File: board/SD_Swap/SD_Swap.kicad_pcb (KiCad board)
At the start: 4 copper layers, 32 x 27 mm, 44 parts, among them J1 USB_C, Q1 Q_Dual_PNP_PNP_E1B1C2E2B2C1, U1 74LVC2G14, U2 RTS5306E, U3 PCB_SD, U4 93AAxxAT, U5 TS3A27518ERTW, U6 SD_SOCKET, U7 AZ1117-3.3, Y1 12MHz

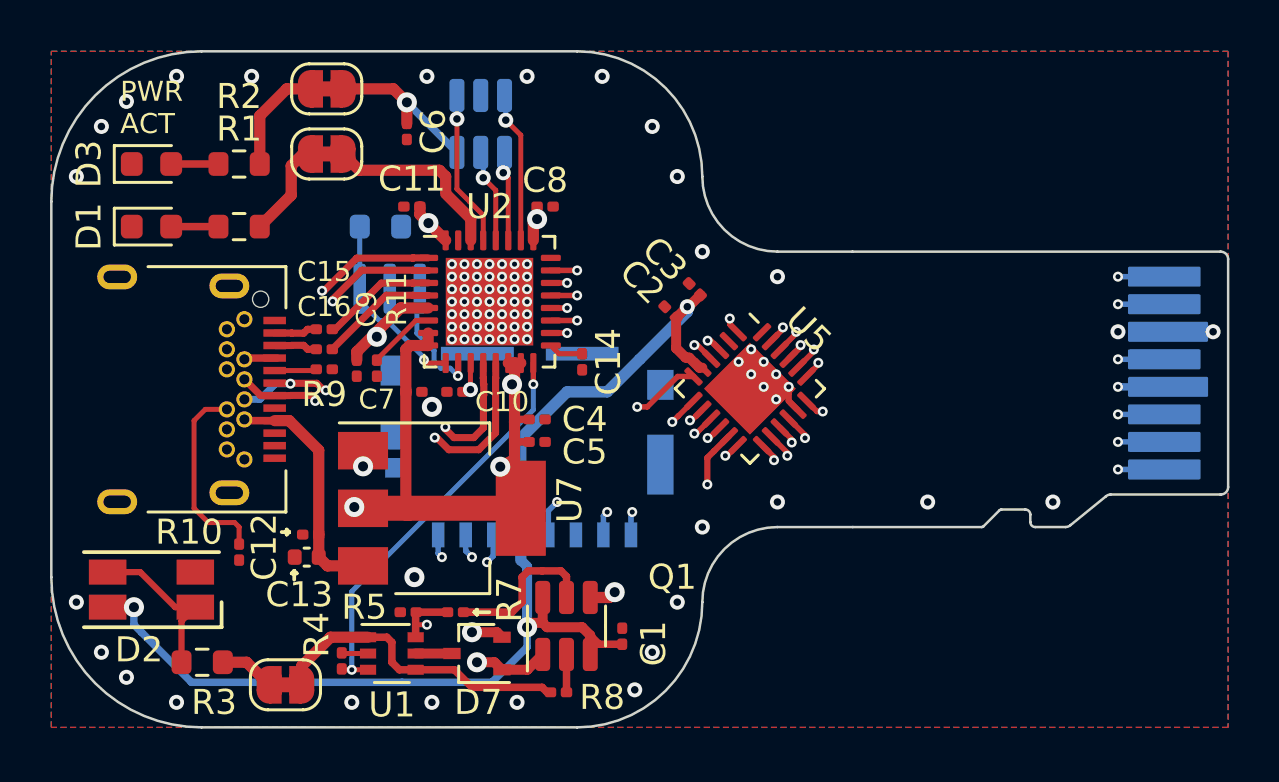
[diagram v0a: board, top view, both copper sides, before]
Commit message: final?
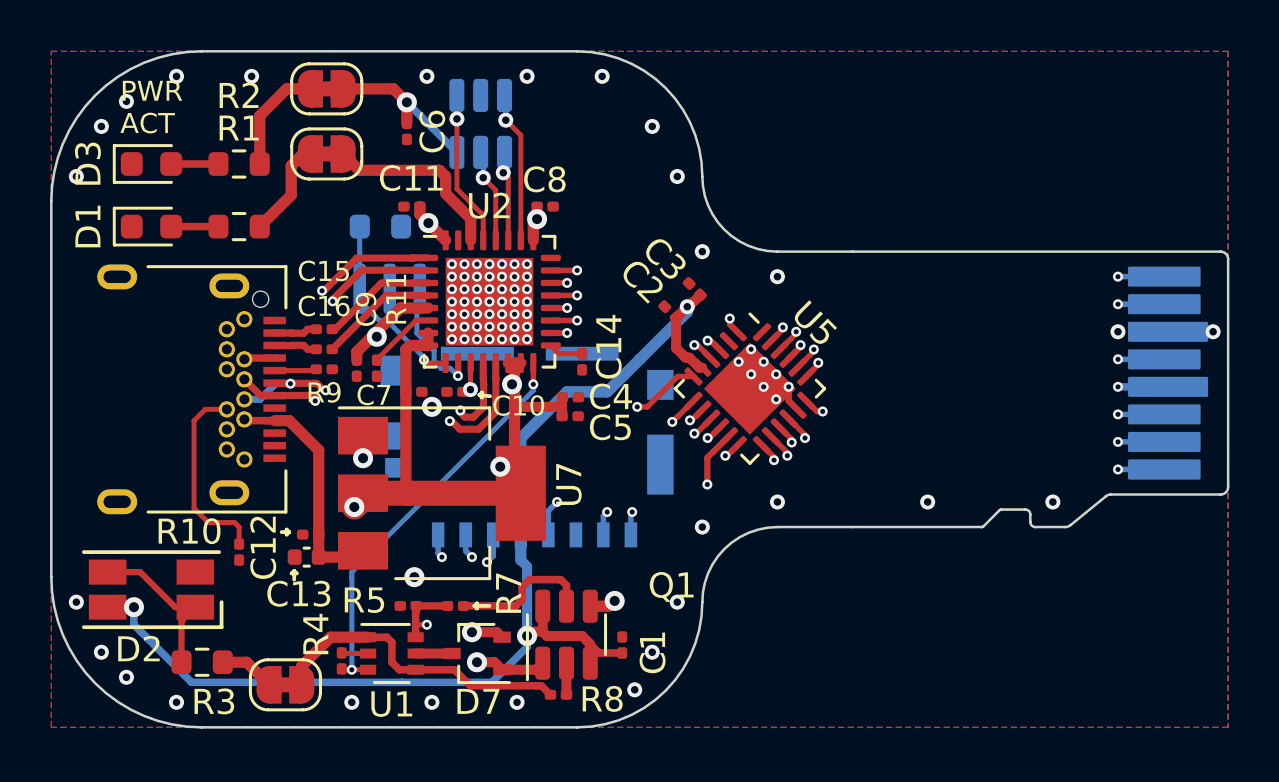
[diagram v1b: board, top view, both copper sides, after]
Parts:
- moved C5 1.67 mm to (111.7, 82.6)
- moved C4 1.59 mm to (111.7, 81.8)
- moved U7 0.60 mm to (106.6, 85.7)
- moved C1 0.35 mm to (113.8, 91.7)
- moved Q1 0.35 mm to (111.6, 91.3)
- moved R5 0.25 mm to (105.3, 90.2)
- moved R7 0.25 mm to (107.1, 90.2)
- moved R8 0.10 mm to (111.3, 93.7)
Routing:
- net /USB+: track 17.3 -> 15.9 mm
- net /USB-: track 15.9 -> 14.7 mm
- net +3.3V: track 32.9 -> 33.7 mm
- net Net-(Q1B-B2): track 6.31 -> 5.77 mm
